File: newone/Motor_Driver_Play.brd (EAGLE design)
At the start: 100 x 80 mm, 88 parts

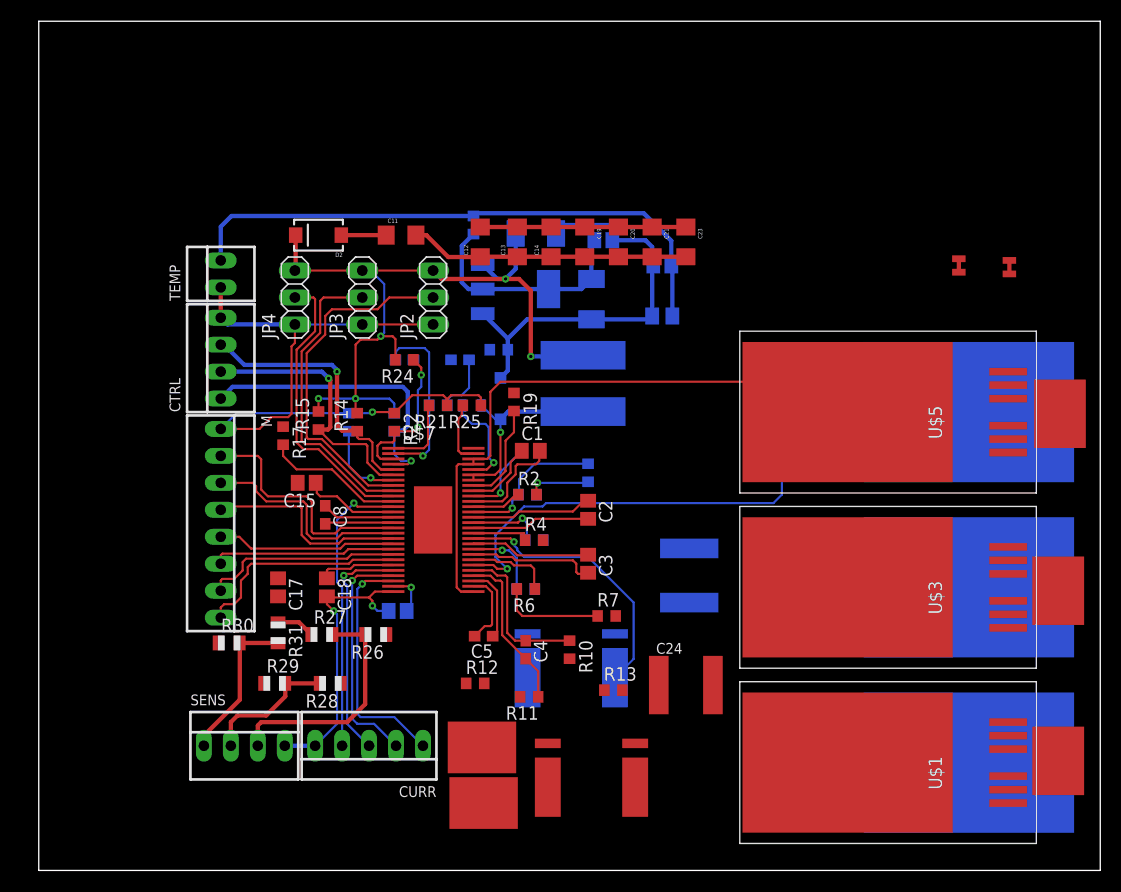
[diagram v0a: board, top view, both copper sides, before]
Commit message: did stuff. So much of stuff
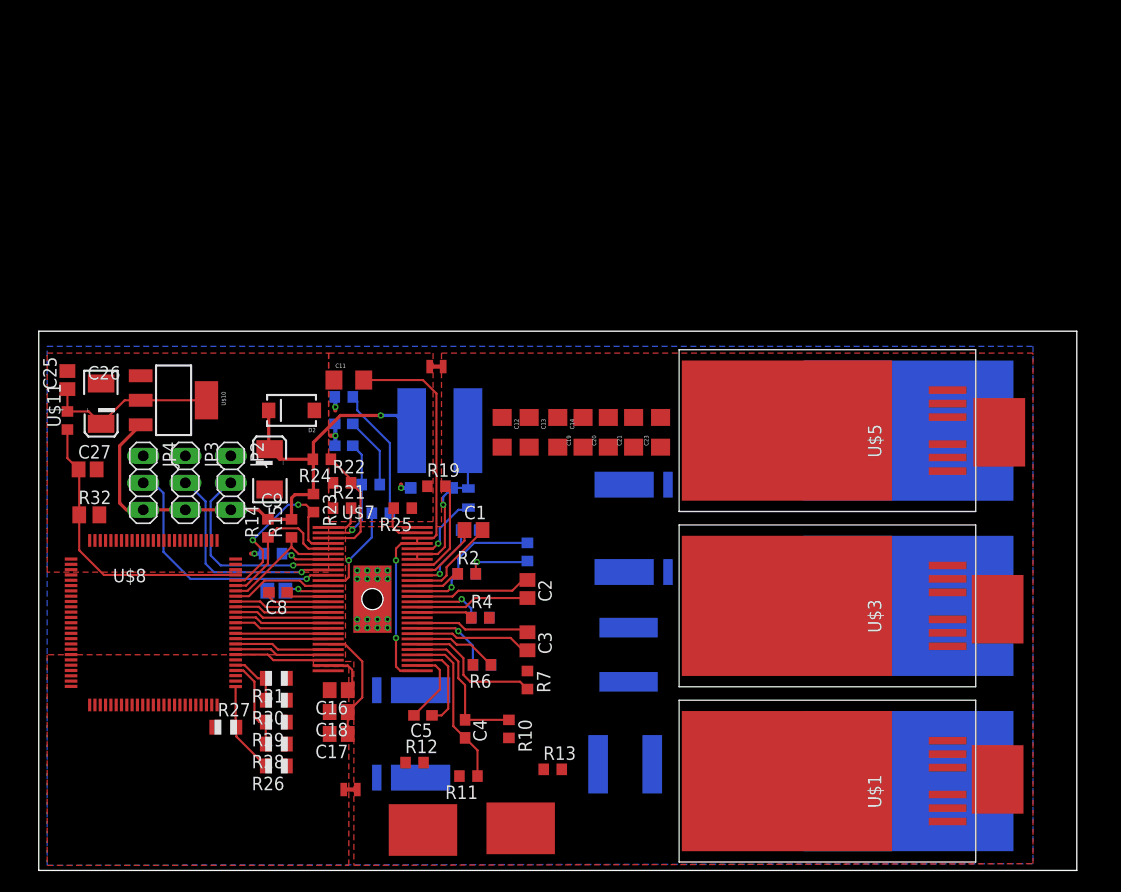
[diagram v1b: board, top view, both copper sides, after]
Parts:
- removed CTRL, SENS: 22-23-2041, con-molex:22-23-2041
- removed CURR: 22-23-2051, con-molex:22-23-2051
- removed M: 22-23-2081, con-molex:22-23-2081
- removed TEMP: 22-23-2021, con-molex:22-23-2021
- added U$8: STM32F4V_100PIN_GENERIC, stm32f4:LQFP100
- moved PT2 75.6 mm to (29.4, 7.62), turned to 270 degrees
- moved C27 57.4 mm to (4.60, 37.8), flipped to the top
- moved R32 57.1 mm to (4.76, 33.5), flipped to the top
- moved PT1 54.8 mm to (37.5, 47.5), turned to 270 degrees
- moved C25 52.2 mm to (2.70, 46.2), flipped to the top, turned to 90 degrees
- moved C26 47.2 mm to (5.87, 44.0), flipped to the top, turned to 270 degrees
- moved U$11 42.5 mm to (2.70, 42.4), flipped to the top, turned to 90 degrees
- moved U$10 33.9 mm to (12.7, 44.3), flipped to the top, turned to 270 degrees
- moved C9 33.5 mm to (21.7, 37.8), flipped to the top, turned to 90 degrees
- moved JP2 25.8 mm to (18.1, 36.5), turned to 270 degrees
- moved JP3 24.1 mm to (13.8, 36.5), turned to 270 degrees
- moved U$18 23.8 mm to (56.0, 32.2), flipped to the bottom, turned to 90 degrees
- moved JP4 22.6 mm to (9.84, 36.5), turned to 270 degrees
- moved C23 18.1 mm to (58.6, 41.3), turned to 90 degrees
- moved C12 18.1 mm to (43.7, 41.3), turned to 270 degrees
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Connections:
- net AGND: now also U$8.PA6; no longer CURR.5, SENS.4
- net DC_CAL: now also U$8.PE12; no longer CURR.4
- net DGND: now also U$8.PB11; no longer CTRL.4, M.1, TEMP.1
- net EN_GATE: now also U$8.PE11; no longer M.2
- net FAULT: now also U$8.PE13; no longer CTRL.2
- net H1: now also U$8.PE10; no longer M.3
- net H2: now also U$8.PE8; no longer M.5
- net H3: now also U$8.PB1; no longer M.7
- net L1: now also U$8.PE9; no longer M.4
- net L2: now also U$8.PE7; no longer M.6
- net L3: now also U$8.PB0; no longer M.8
- net OCTW: now also U$8.PE14; no longer CTRL.3
- net PWRGD: now also U$8.PE15; no longer CTRL.1
- net REF: now also U$8.PC5; no longer CURR.3
- net SENS1: now also U$8.PA3; no longer SENS.3
- net SENS2: now also U$8.PA4; no longer SENS.2
- net SENS3: now also U$8.PA5; no longer SENS.1
- net SO1: now also U$8.PC4; no longer CURR.2
- net SO2: now also U$8.PA7; no longer CURR.1
- net TEMP: now also U$8.PB10; no longer TEMP.2
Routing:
- net DGND: track 110.0 -> 6.30 mm, vias 1 -> 4
- net VCC: track 84.6 -> 38.6 mm, vias 0 -> 2
- net GND: track 45.0 -> 0.00 mm, vias 1 -> 16
- net AGND: track 31.0 -> 0.00 mm, vias 2 -> 0
- net H3_LOW: track 42.9 -> 13.1 mm, vias 1 -> 0
- net TEMP: track 54.3 -> 27.5 mm
- net +5V: track 74.7 -> 53.2 mm, vias 5 -> 1
- net DC_CAL: track 27.6 -> 9.53 mm, vias 1 -> 0
- net FAULT: track 26.0 -> 11.6 mm, vias 1 -> 0
- net SO2: track 22.9 -> 8.94 mm, vias 1 -> 0
- net EN_GATE: track 22.8 -> 8.94 mm
- net M_PWM: track 33.1 -> 19.2 mm, vias 0 -> 1
- net SENS1: track 22.5 -> 8.65 mm
- net SO1: track 22.3 -> 8.94 mm, vias 1 -> 0
- net REF: track 21.9 -> 8.94 mm, vias 1 -> 0
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- added copper zone on layer 1, net AGND
- added copper zone on layer 1, net DGND
- added copper zone on layer 1, net GND
- added copper zone on layer 16, net GND
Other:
- board size 100 x 80 mm -> 97.8 x 50.8 mm

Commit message: work damnit
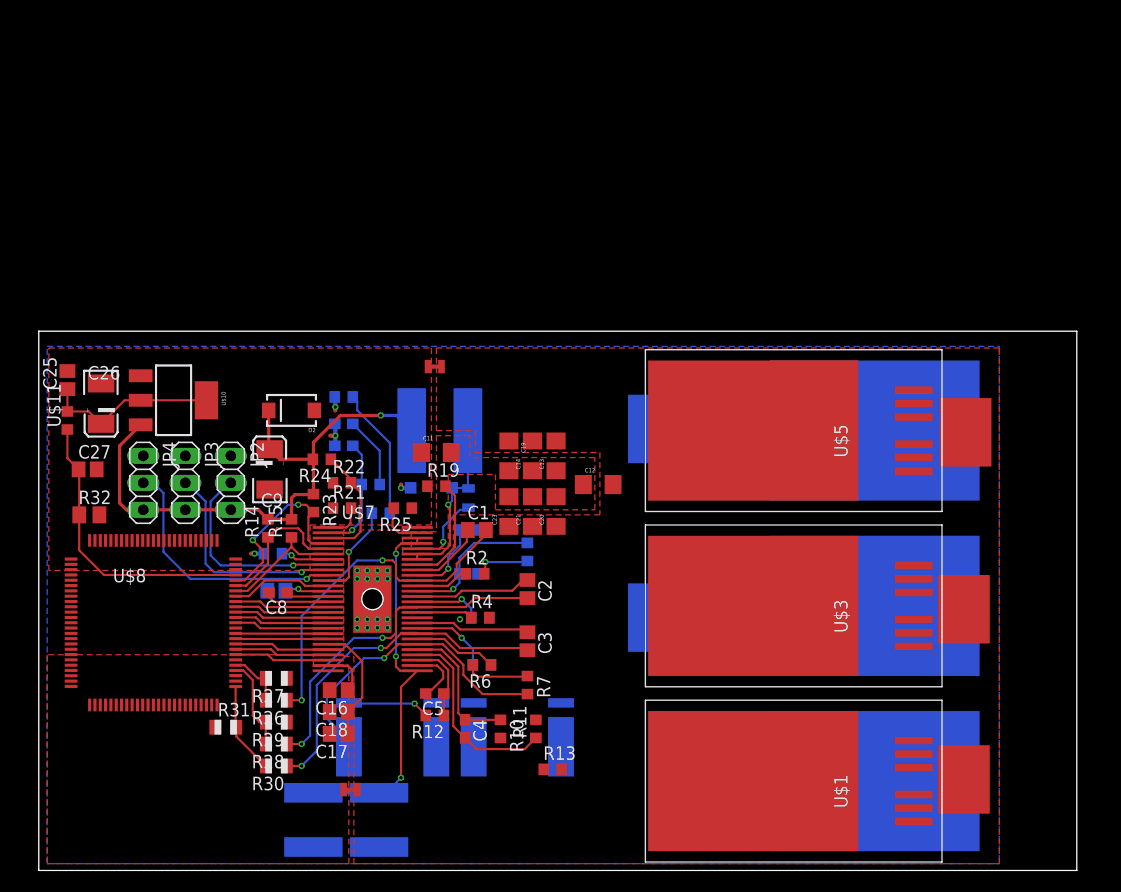
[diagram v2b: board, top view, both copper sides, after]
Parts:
- moved U$12 39.7 mm to (57.9, 41.6), flipped to the bottom, turned to 90 degrees
- moved C22 33.5 mm to (25.9, 4.76)
- moved U$13 29.5 mm to (57.9, 23.8), flipped to the bottom, turned to 90 degrees
- moved C24 23.8 mm to (32.1, 4.76), turned to 90 degrees
- moved U$18 22.5 mm to (45.1, 12.5), turned to 0 degrees
- moved C23 16.1 mm to (44.3, 33.8)
- moved C21 12.1 mm to (46.5, 33.8)
- moved C11 10.7 mm to (37.5, 39.4)
- moved C12 10.3 mm to (52.7, 36.4), turned to 0 degrees
- moved C20 8.94 mm to (48.7, 33.8)
- moved R11 7.75 mm to (46.8, 13.3), turned to 90 degrees
- moved C19 7.33 mm to (44.3, 39.1), turned to 270 degrees
- moved R27 6.62 mm to (22.4, 18.1), turned to 180 degrees
- moved R31 6.62 mm to (17.6, 13.5), turned to 0 degrees
- moved R26 6.19 mm to (22.4, 16.0)
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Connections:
- net SENS1: now also U$8.PA5; no longer U$8.PA3
- net SENS3: now also U$8.PA3; no longer U$8.PA5
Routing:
- net H1_VS: track 8.65 -> 33.0 mm, vias 0 -> 2
- net H2_VS: track 10.7 -> 32.5 mm, vias 0 -> 2
- net H3_VS: track 11.0 -> 32.2 mm, vias 0 -> 2
- net H3_LOW: track 13.1 -> 29.1 mm, vias 0 -> 1
- net N$25: track 0.00 -> 7.75 mm, vias 0 -> 1
- net N$6: track 0.00 -> 6.05 mm
- net SENS3: track 5.42 -> 8.65 mm
- net SENS1: track 8.65 -> 5.42 mm
- net N$23: track 15.3 -> 18.5 mm
- net VCC: track 38.6 -> 35.5 mm, vias 2 -> 3
- net N$11: track 7.60 -> 5.56 mm
- net N$22: track 14.4 -> 13.2 mm
- net N$24: track 8.94 -> 7.77 mm
- net N$2: track 5.96 -> 5.16 mm
- net GL_A: track 4.29 -> 5.09 mm
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- added copper zone on layer 1, net VCC

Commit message: things happened. Board mostly done
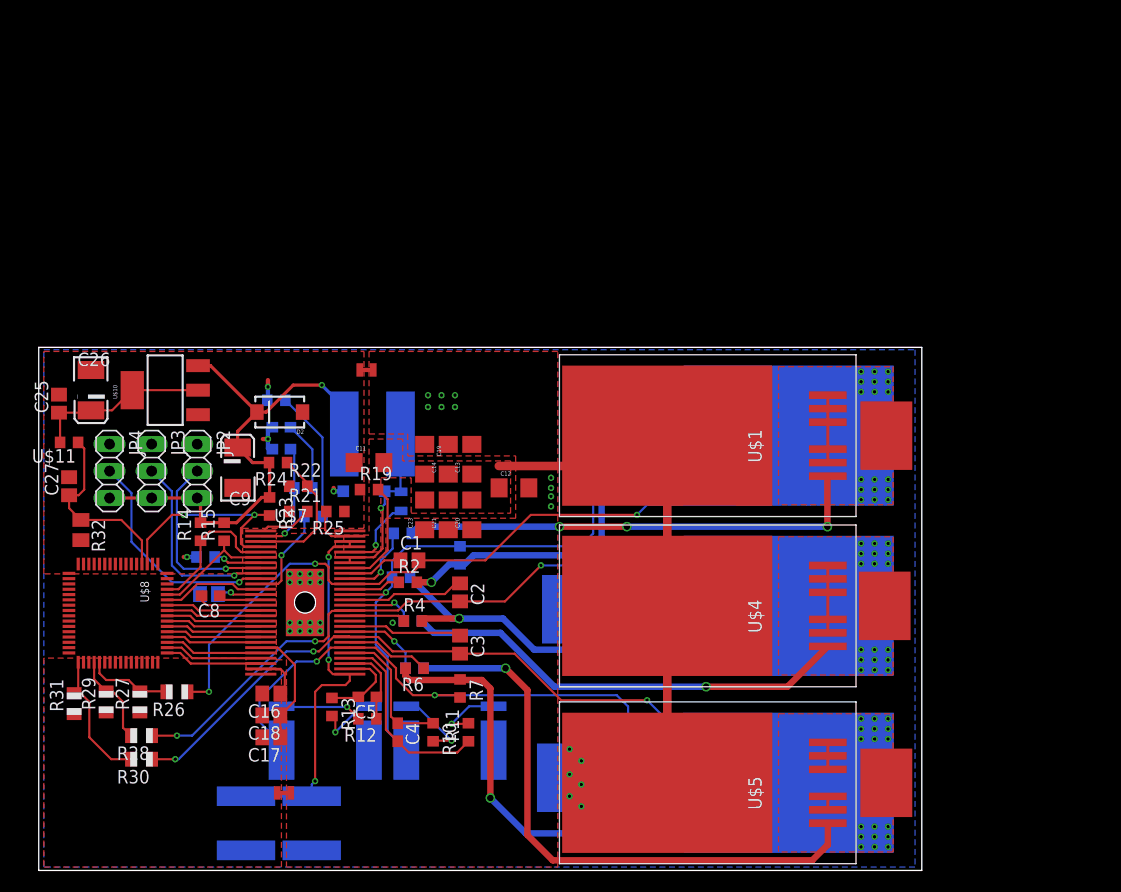
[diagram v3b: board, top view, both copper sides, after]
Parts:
- R1, R2, R3, R4, R5, R6: value 4.7K -> 1
- R7, R8, R9: value 39K -> 0
- U$8: value STM32F4V_100PIN_GENERIC -> STM32F4R_64PIN_FOXCAR; device stm32f4:LQFP100 -> stm32f4:LQFP64
- moved U$15 50.0 mm to (49.4, 8.73), flipped to the bottom
- moved U$12 39.9 mm to (79.9, 8.26), flipped to the top
- moved U$16 37.3 mm to (49.8, 24.6), flipped to the bottom
- moved U$5 34.2 mm to (60.5, 8.26)
- moved U$6 34.2 mm to (69.4, 8.26)
- moved U$1 33.5 mm to (60.5, 41.0)
- moved U$2 33.5 mm to (69.4, 41.0)
- moved U$14 33.2 mm to (79.9, 41.0)
- moved U$13 21.8 mm to (79.7, 24.9), flipped to the top
- moved R13 21.6 mm to (27.6, 15.4), turned to 270 degrees
- moved U$4 17.0 mm to (60.5, 24.9), flipped to the top
- moved R29 16.1 mm to (6.35, 15.9), turned to 90 degrees
- moved R31 14.5 mm to (3.33, 15.7), turned to 90 degrees
- moved R27 13.0 mm to (9.53, 15.9), turned to 90 degrees
- moved R28 12.7 mm to (9.68, 12.7)
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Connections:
- net AGND: now also U$8.22; no longer U$8.PA6
- net DC_CAL: now also U$8.43; no longer U$8.PE12
- net DGND: now also U$8.53; no longer U$8.PB11
- net EN_GATE: now also U$8.42; no longer U$8.PE11
- net FAULT: now also U$8.44; no longer U$8.PE13
- net H1: now also U$8.41; no longer U$8.PE10
- net H2: now also U$8.39; no longer U$8.PE8
- net H3: now also U$8.37; no longer U$8.PB1
- net L1: now also U$8.40; no longer U$8.PE9
- net L2: now also U$8.38; no longer U$8.PE7
- net L3: now also U$8.36; no longer U$8.PB0
- net OCTW: now also U$8.45; no longer U$8.PE14
- net PWRGD: now also U$8.51; no longer U$8.PE15
- net REF: now also U$8.35; no longer U$8.PC5
- net SENS1: now also U$8.21; no longer U$8.PA5
- net SENS2: now also U$8.20; no longer U$8.PA4
- net SENS3: now also U$8.17; no longer U$8.PA3
- net SO1: now also U$8.34; no longer U$8.PC4
- net SO2: now also U$8.33; no longer U$8.PA7
- net TEMP: now also U$8.52; no longer U$8.PB10
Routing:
- net N$5: track 0.00 -> 56.2 mm, vias 0 -> 1
- net VCC: track 35.5 -> 86.8 mm, vias 3 -> 9
- net H1_VS: track 33.0 -> 81.4 mm, vias 2 -> 21
- net H2_VS: track 32.5 -> 78.6 mm, vias 2 -> 21
- net H1_LOW: track 13.7 -> 58.8 mm
- net N$1: track 0.00 -> 44.2 mm, vias 0 -> 3
- net N$4: track 0.00 -> 42.4 mm, vias 0 -> 1
- net H3_VS: track 32.2 -> 74.3 mm, vias 2 -> 21
- net H3_LOW: track 29.1 -> 57.5 mm, vias 1 -> 2
- net N$6: track 6.05 -> 34.3 mm, vias 0 -> 1
- net N$3: track 0.00 -> 27.1 mm, vias 0 -> 1
- net N$2: track 5.16 -> 27.1 mm
- net TEMP: track 27.5 -> 17.9 mm
- net N$9: track 0.00 -> 7.38 mm, vias 0 -> 1
- net N$33: track 0.00 -> 6.25 mm, vias 0 -> 1
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- added copper zone on layer 1, net H1_VS
- added copper zone on layer 1, net H2_VS
- added copper zone on layer 1, net H3_VS
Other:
- board size 97.8 x 50.8 mm -> 83.2 x 49.3 mm
